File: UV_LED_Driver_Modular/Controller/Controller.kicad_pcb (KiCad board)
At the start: 2 copper layers, 68.6 x 39.4 mm, 20 parts, among them J1 Barrel_Jack, J2 Conn_01x05, J3 Conn_02x06_Odd_Even, J4 Conn_01x03, Q1 Q_NPN_BCE, Q2 Q_NPN_BCE, Q3 Q_NPN_BCE, SW1 SW_SPST, U1 STM32L011D4Px, U2 MCP1703A-3302_SOT223

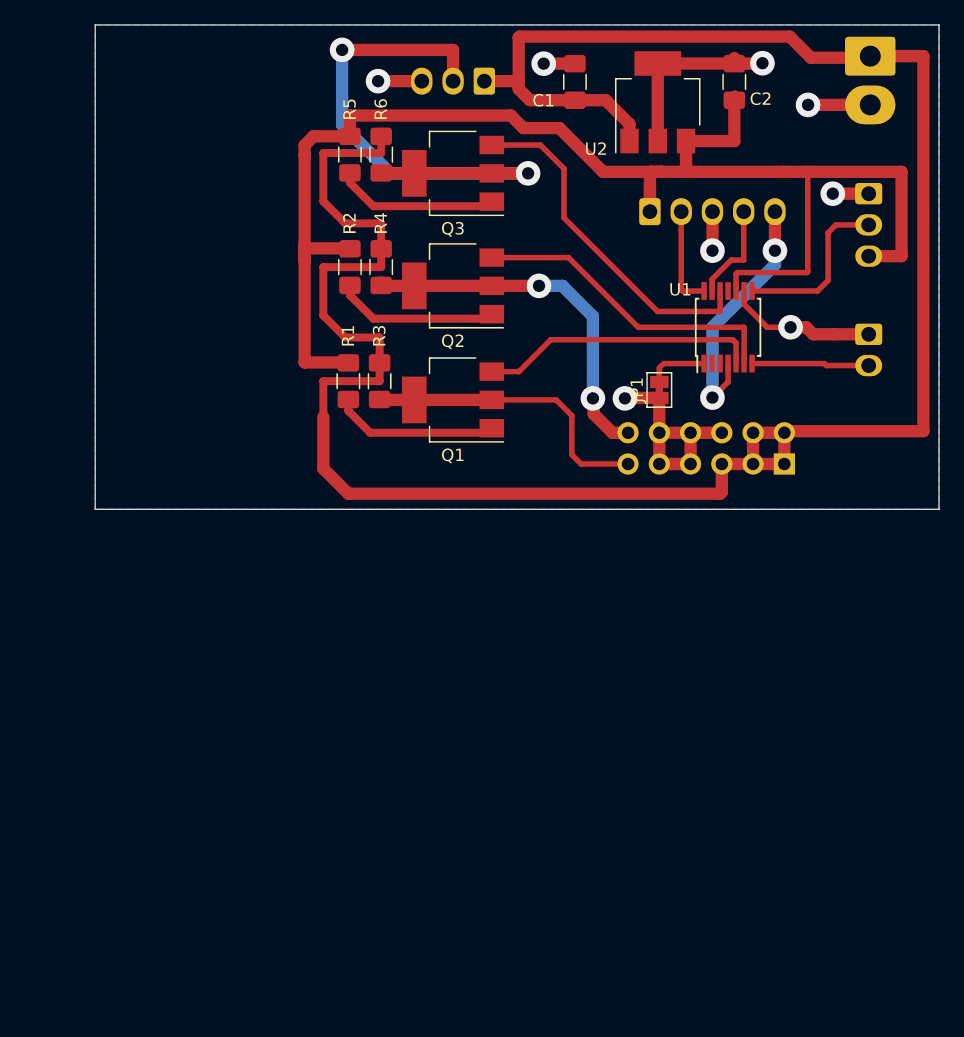
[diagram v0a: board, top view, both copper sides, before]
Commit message: docs update
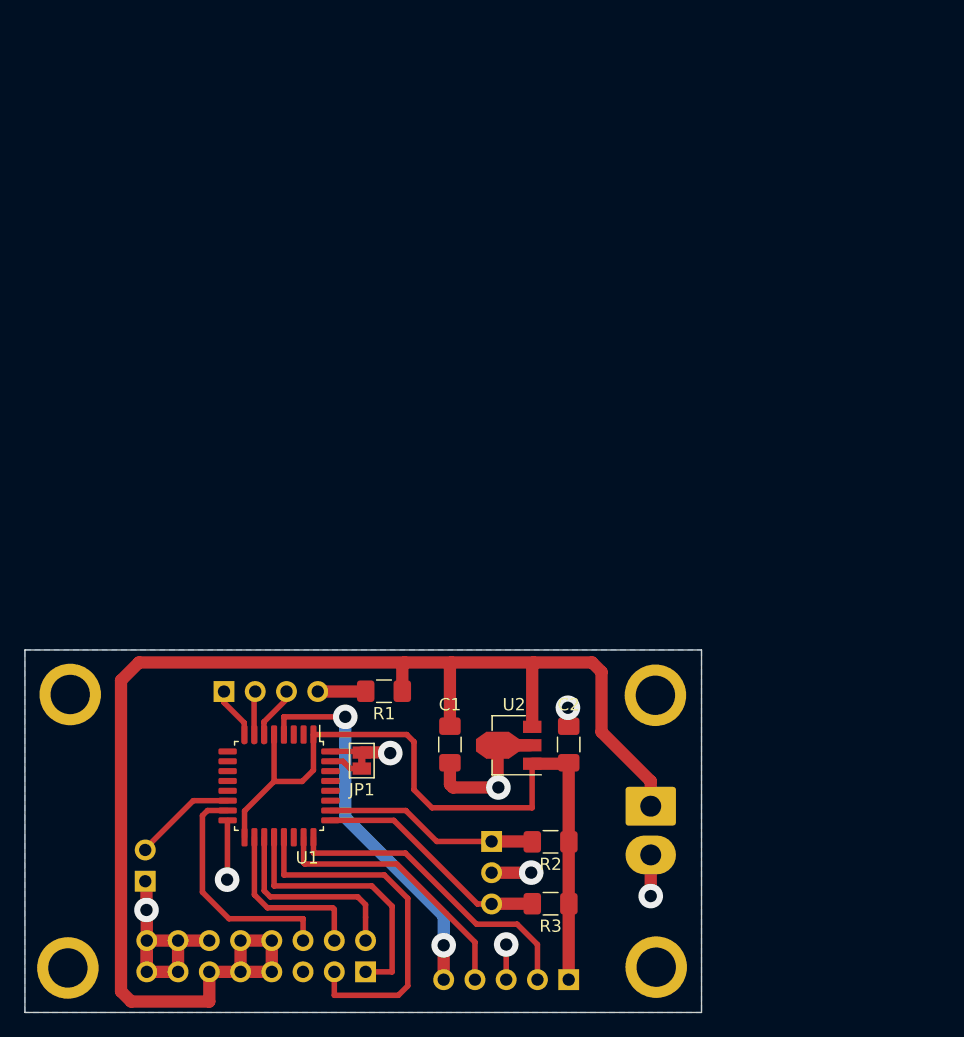
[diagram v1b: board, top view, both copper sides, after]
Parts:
- removed J4: Conn_01x03, Connector_Molex:Molex_KK-254_AE-6410-03A_1x03_P2.54mm_Vertical
- removed Q1, Q2, Q3: Q_NPN_BCE, Package_TO_SOT_SMD:SOT-223-3_TabPin2
- removed R4, R6: 2K2, Resistor_SMD:R_1206_3216Metric_Pad1.42x1.75mm_HandSolder
- removed R5: 1K, Resistor_SMD:R_1206_3216Metric_Pad1.42x1.75mm_HandSolder
- removed RV1: B10K, Connector_Molex:Molex_KK-254_AE-6410-03A_1x03_P2.54mm_Vertical
- added D1: LED_RGBA, Connector_PinHeader_2.54mm:PinHeader_1x04_P2.54mm_Vertical, B.Cu at (61.3, 105.0)
- added REF**: MountingHole_3.2mm_M3, MountingHole:MountingHole_3.2mm_M3, F.Cu at (48.6, 127.4)
- added REF**: MountingHole_3.2mm_M3, MountingHole:MountingHole_3.2mm_M3, F.Cu at (96.3, 105.3)
- added REF**: MountingHole_3.2mm_M3, MountingHole:MountingHole_3.2mm_M3, F.Cu at (48.8, 105.2)
- added REF**: MountingHole_3.2mm_M3, MountingHole:MountingHole_3.2mm_M3, F.Cu at (96.4, 127.4)
- added SW2: Rotary_Encoder, Connector_PinHeader_2.54mm:PinHeader_1x03_P2.54mm_Vertical, B.Cu at (83.0, 117.2)
- J2: footprint Connector_Molex:Molex_KK-254_AE-6410-05A_1x05_P2.54mm_Vertical -> Connector_PinHeader_2.54mm:PinHeader_1x05_P2.54mm_Vertical
- J3: value Conn_02x06_Odd_Even -> Conn_02x08_Odd_Even; footprint Connector_IDC:IDC-Header_2x06_P2.54mm_Vertical -> Connector_PinHeader_2.54mm:PinHeader_2x08_P2.54mm_Vertical
- R1: value 1K -> 2K2
- R2: value 1K -> 10K
- R3: value 2K2 -> 10K
- SW1: footprint Connector_Molex:Molex_KK-254_AE-6410-02A_1x02_P2.54mm_Vertical -> Connector_PinHeader_2.54mm:PinHeader_1x02_P2.54mm_Vertical
- U1: value STM32L011D4Px -> STM32F051K8Tx; footprint Package_SO:TSSOP-14_4.4x5mm_P0.65mm -> Package_QFP:LQFP-32_7x7mm_P0.8mm
- U2: value MCP1703A-3302_SOT223 -> L78L33_SOT89; footprint Package_TO_SOT_SMD:SOT-223-3_TabPin2 -> Package_TO_SOT_SMD:SOT-89-3
- moved SW1 73.7 mm to (54.9, 120.4), turned to 0 degrees
- moved J1 63.5 mm to (95.9, 114.3)
- moved J2 62.8 mm to (89.3, 128.4), turned to 90 degrees
- moved C2 55.5 mm to (89.3, 109.3)
- moved C1 54.8 mm to (79.6, 109.3), turned to 270 degrees
- moved U2 53.6 mm to (84.8, 109.3), turned to 180 degrees
- moved J3 53.5 mm to (72.8, 127.8)
- moved U1 52.2 mm to (65.7, 112.6), turned to 270 degrees
- moved R2 49.5 mm to (87.8, 117.2), turned to 180 degrees
- moved R3 44.7 mm to (87.8, 122.2), turned to 180 degrees
- moved JP1 38.6 mm to (72.5, 110.6), turned to 270 degrees
- moved R1 25.4 mm to (74.3, 105.0), turned to 180 degrees
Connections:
- C1 pad 1: +5V -> VPP
- J1 pad 1: +5V -> VPP
- J3 pad 1: +5V -> /LED_PWM_OUT2
- J3 pad 10: GNDS -> VPP
- J3 pad 11: /UV_PWM_OUT -> VPP
- J3 pad 12: /LED_PWM_OUT -> GNDS
- J3 pad 2: +5V -> /LED_PWM_OUT3
- J3 pad 3: +5V -> /LED_PWM_OUT1
- J3 pad 4: +5V -> /LED_PWM_OUT4
- J3 pad 5: +5V -> Net-(J3-Pad5)
- J3 pad 6: GNDS -> /LED_PWM_OUT5
- J3 pad 7: GNDS -> VPP
- J3 pad 8: GNDS -> VPP
- J3 pad 9: GNDS -> VPP
- R1 pad 1: +3V3 -> VPP
- R2 pad 2: Net-(Q2-Pad1) -> /LED_Controller_Module/ENC_A
- R3 pad 1: +5V -> +3V3
- R3 pad 2: /UV_PWM_OUT -> /LED_Controller_Module/ENC_B
- SW1 pad 2: /LED_Controller_Module/LID_SW -> /LED_Controller_Module/ENABLE_LED
- U1 pad 1: Net-(JP1-Pad2) -> +3V3
- U1 pad 10: +3V3 -> Net-(U1-Pad10)
- U1 pad 12: /LED_Controller_Module/STATUS_PWM -> Net-(U1-Pad12)
- U1 pad 13: /LED_Controller_Module/SWDIO -> Net-(U1-Pad13)
- U1 pad 14: /LED_Controller_Module/SWCLK -> /LED_Controller_Module/ENABLE_LED
- U1 pad 5: /LED_Controller_Module/UV_LED_PWM -> +3V3
- U1 pad 6: /LED_Controller_Module/LED_PWM -> /LED_Controller_Module/STATUS_BLUE
- U1 pad 7: /LED_Controller_Module/LID_SW -> /LED_Controller_Module/STATUS_GREEN
- U1 pad 8: /LED_Controller_Module/LED_ADC -> /LED_Controller_Module/STATUS_RED
- U1 pad 9: GNDS -> Net-(U1-Pad9)
- U2 pad 1: +5V -> +3V3
- U2 pad 3: +3V3 -> VPP
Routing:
- net +5V: track 190.5 -> 0.00 mm
- net VPP: track 0.00 -> 113.6 mm
- net +3V3: track 119.6 -> 62.7 mm
- net /STATUS_PWM_OUT: track 46.3 -> 0.00 mm, vias 2 -> 0
- net /LED_PWM_OUT: track 29.5 -> 0.00 mm, vias 2 -> 0
- net /LED_PWM_OUT1: track 0.00 -> 29.2 mm
- net /LED_Controller_Module/STATUS_PWM: track 28.2 -> 0.00 mm
- net /LED_Controller_Module/LED_PWM: track 25.8 -> 0.00 mm
- net /UV_PWM_OUT: track 24.1 -> 0.00 mm
- net /LED_Controller_Module/UV_LED_PWM: track 22.7 -> 0.00 mm
- net /LED_PWM_OUT2: track 0.00 -> 21.7 mm
- net /LED_Controller_Module/ENC_B: track 0.00 -> 19.4 mm
- net /LED_PWM_OUT5: track 0.00 -> 19.3 mm
- net /LED_Controller_Module/ENC_A: track 0.00 -> 17.7 mm
- net /LED_Controller_Module/SWCLK: track 8.63 -> 25.4 mm
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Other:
- board size 68.6 x 39.4 mm -> 55 x 29.5 mm
